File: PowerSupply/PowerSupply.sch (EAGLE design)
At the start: 19 parts, among them Q2 DMMT5401, Q3 DMG2305UX

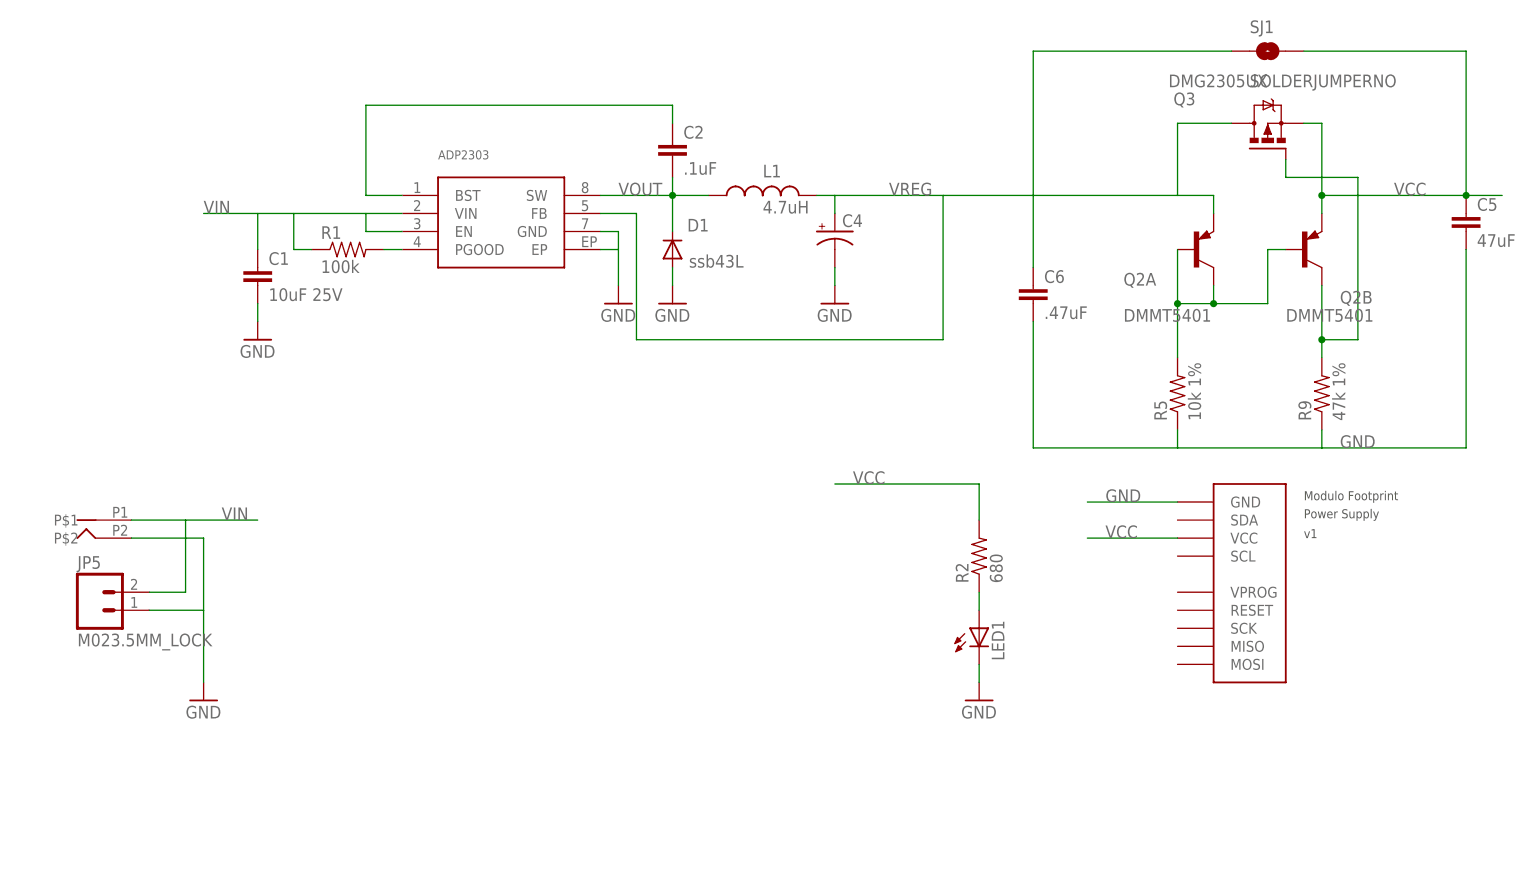
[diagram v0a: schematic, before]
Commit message: various minor changes
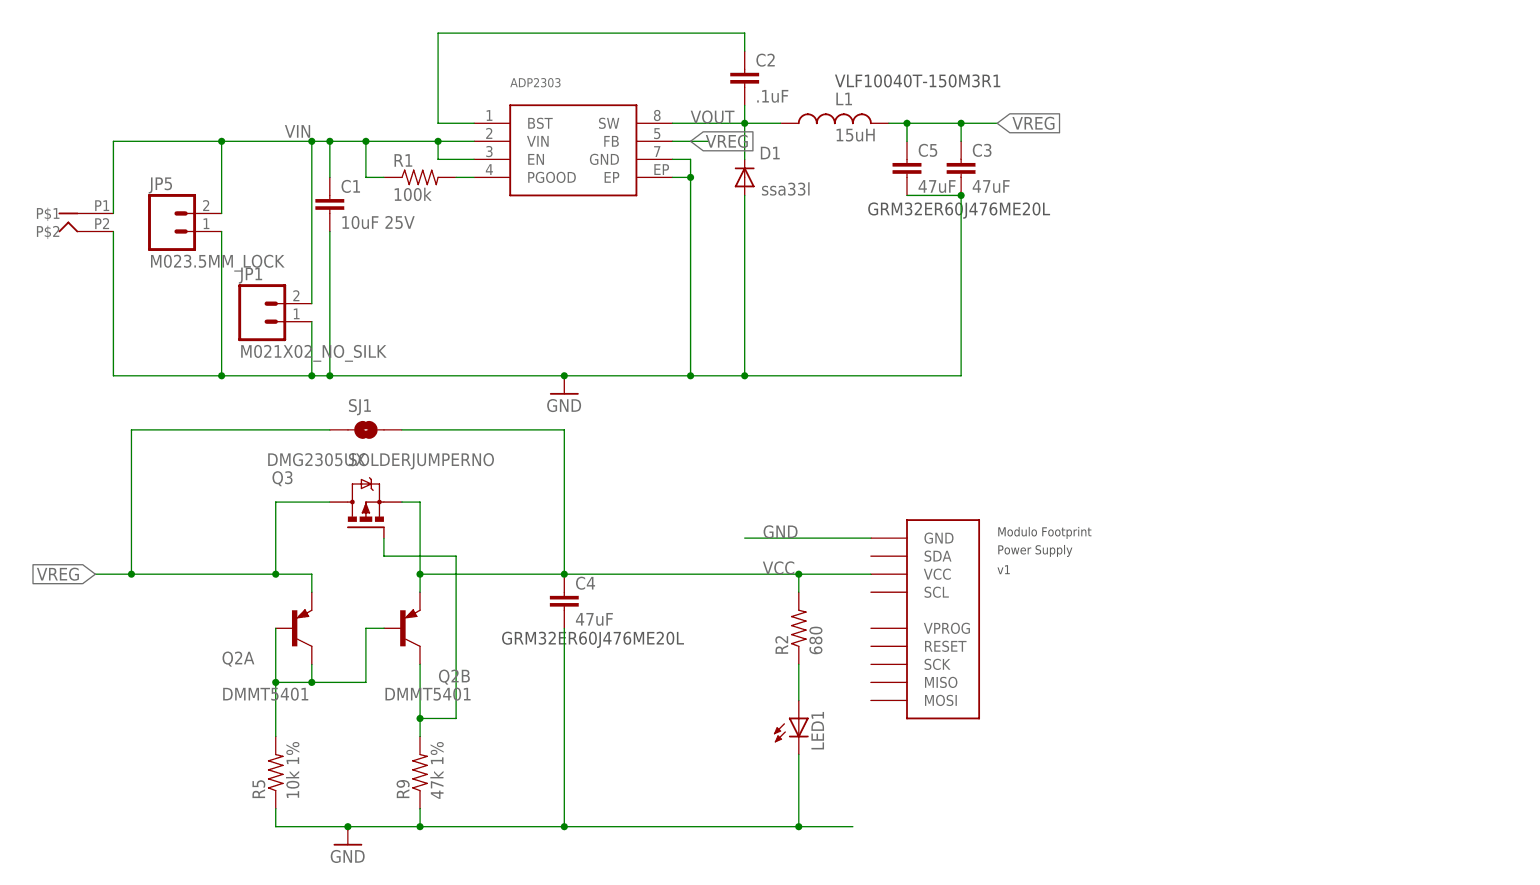
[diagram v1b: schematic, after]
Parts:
- removed C6: .47uF, SparkFun-Capacitors:CAP0805
- added C3: 47uF, SparkFun-Capacitors:CAP1210
- added JP1: M021X02_NO_SILK, SparkFun-Connectors:M021X02_NO_SILK
- C4: value (none) -> 47uF; device adafruit:CPOL-USB -> SparkFun-Capacitors:CAP1210
- C5: device SparkFun-Capacitors:CAP0805 -> SparkFun-Capacitors:CAP1210
- D1: value ssb43L -> ssa33l; device SparkFun-DiscreteSemi:DIODESMB -> SparkFun-DiscreteSemi:DIODESMA
- L1: value 4.7uH -> 15uH
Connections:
- net GND: now also C3.2, C4.2, JP1.1; no longer C4.-, C6.2
- net VCC: now also C4.1; no longer C5.1
- net VIN: now also JP1.2
- net VREG: now also C3.1, C5.1; no longer C4.+, C6.1
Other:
- note added: "GRM32ER60J476ME20L"
- note added: "VLF10040T-150M3R1"
- moved on the sheet: C1, C2, C5, D1, JP5, L1, LED1, Q2A, Q2B, Q3, R1, R2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
